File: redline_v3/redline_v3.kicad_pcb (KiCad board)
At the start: 2 copper layers, 89.1 x 94.5 mm, 67 parts, among them J1 Conn_01x10_Socket, J2 Conn_01x10_Socket

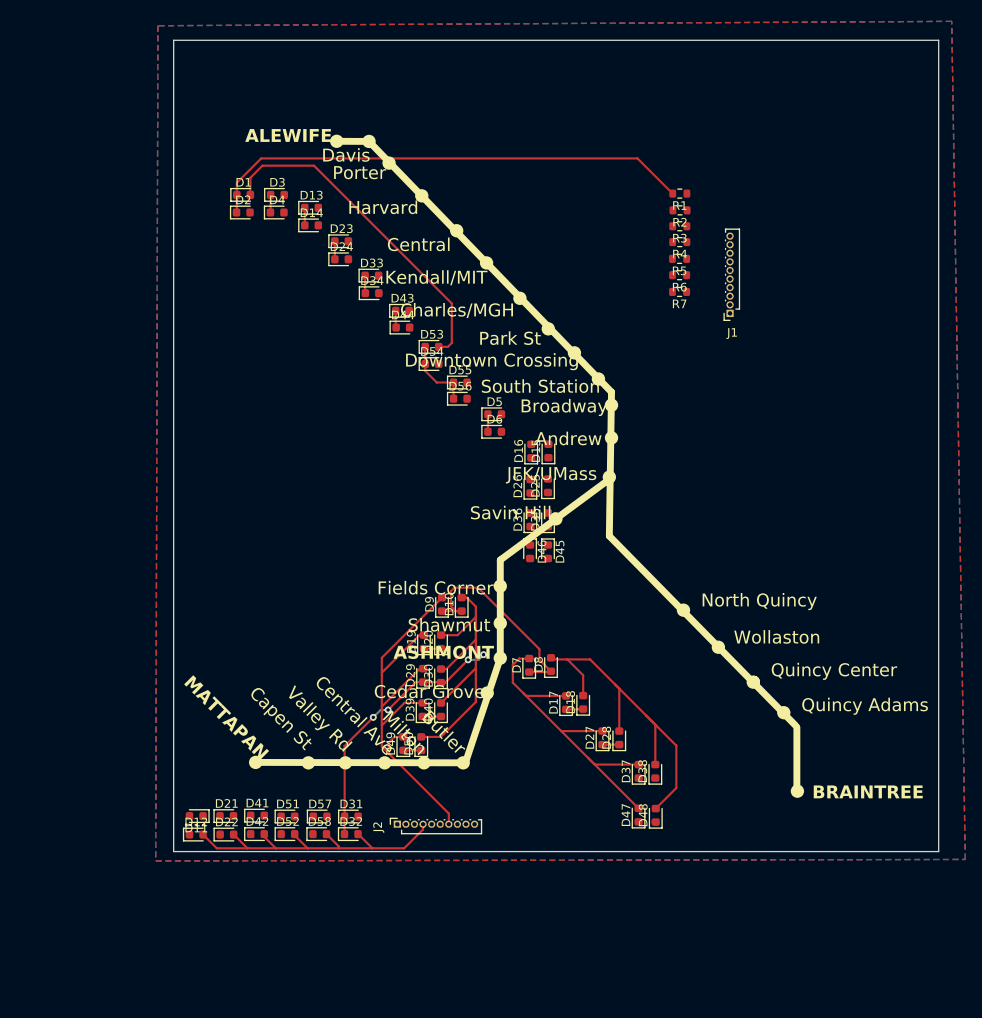
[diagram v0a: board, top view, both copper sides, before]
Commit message: V3 with Gia layout
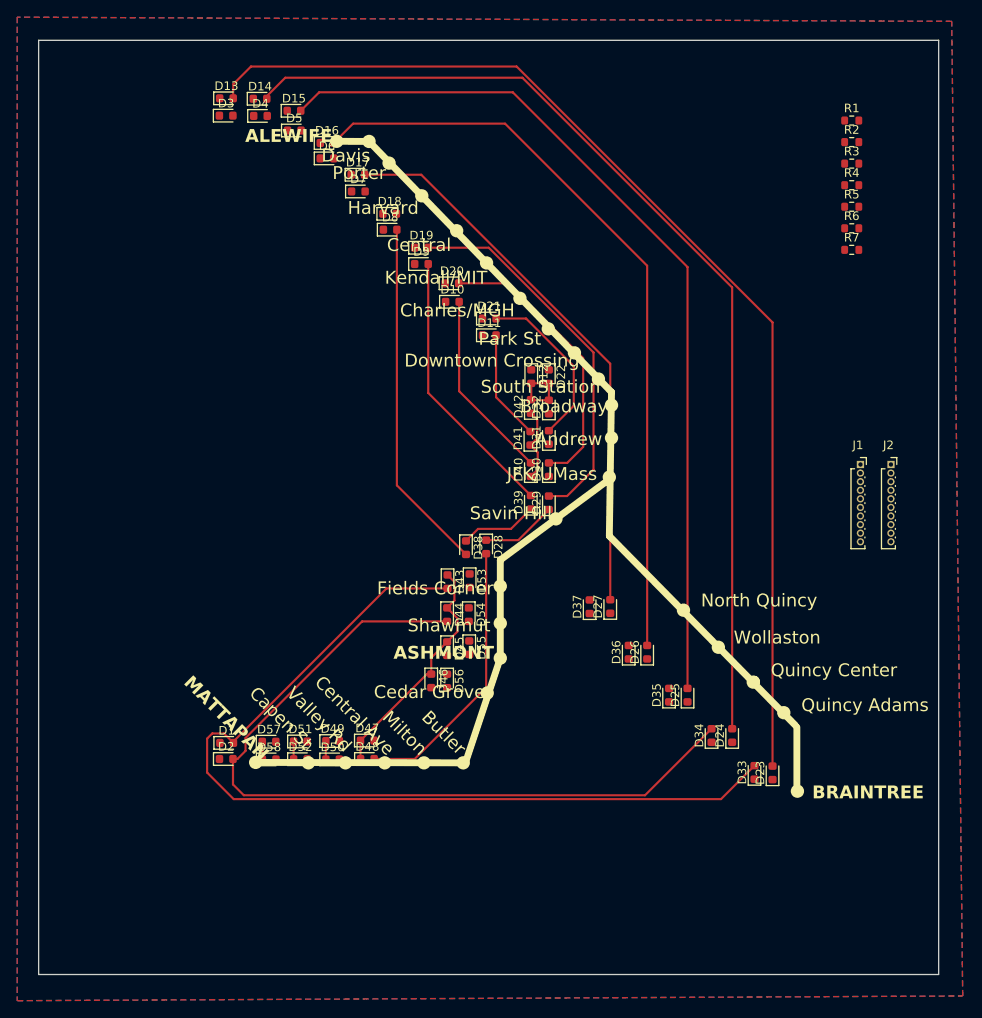
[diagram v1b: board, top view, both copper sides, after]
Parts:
- moved D23 79.7 mm to (218.7, 137.6), turned to 90 degrees
- moved D33 73.0 mm to (216.6, 137.5), turned to 90 degrees
- moved D24 71.7 mm to (213.9, 133.2), turned to 90 degrees
- moved J2 71.1 mm to (232.4, 101.7), turned to 0 degrees
- moved D17 66.1 mm to (170.4, 67.9), turned to 0 degrees
- moved D12 66.1 mm to (190.6, 91.4), turned to -90 degrees
- moved D11 65.6 mm to (185.7, 86.6), turned to 0 degrees
- moved D21 65.5 mm to (185.7, 84.7)
- moved D22 65.2 mm to (192.6, 91.4), turned to -90 degrees
- moved D34 64.9 mm to (211.6, 133.2), turned to 90 degrees
- moved D1 63.9 mm to (155.1, 134.1)
- moved D2 63.7 mm to (155.0, 135.9)
- moved D18 61.2 mm to (174.1, 72.5), turned to 0 degrees
- moved D42 59.1 mm to (190.5, 94.9), turned to 90 degrees
- moved D7 58.7 mm to (170.4, 69.8), turned to 0 degrees
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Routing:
- net /1: track 0.00 -> 211.9 mm
- net /0: track 39.0 -> 236.2 mm
- net /2: track 0.00 -> 103.5 mm
- net /3: track 0.00 -> 88.5 mm
- net Net-(D1-K): track 57.1 -> 0.00 mm
- net /8: track 0.00 -> 32.9 mm
- net /9: track 39.2 -> 8.06 mm
- net /5: track 44.0 -> 73.3 mm
- net Net-(D10-K): track 28.8 -> 0.00 mm
- net Net-(D43-K): track 4.46 -> 31.8 mm
- net Net-(D23-K): track 35.0 -> 8.78 mm, vias 4 -> 0
- net /4: track 41.5 -> 65.3 mm
- net /6: track 55.0 -> 76.3 mm
- net /7: track 37.4 -> 55.5 mm
- net Net-(D33-K): track 4.57 -> 17.8 mm
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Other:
- board size 89.1 x 94.5 mm -> 104.8 x 108.8 mm
